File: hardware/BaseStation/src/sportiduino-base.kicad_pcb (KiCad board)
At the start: 2 copper layers, 76.8 x 44.7 mm, 38 parts, among them SW1 SW_Reed, X1 Battery, X2 Prog, X3 RC522

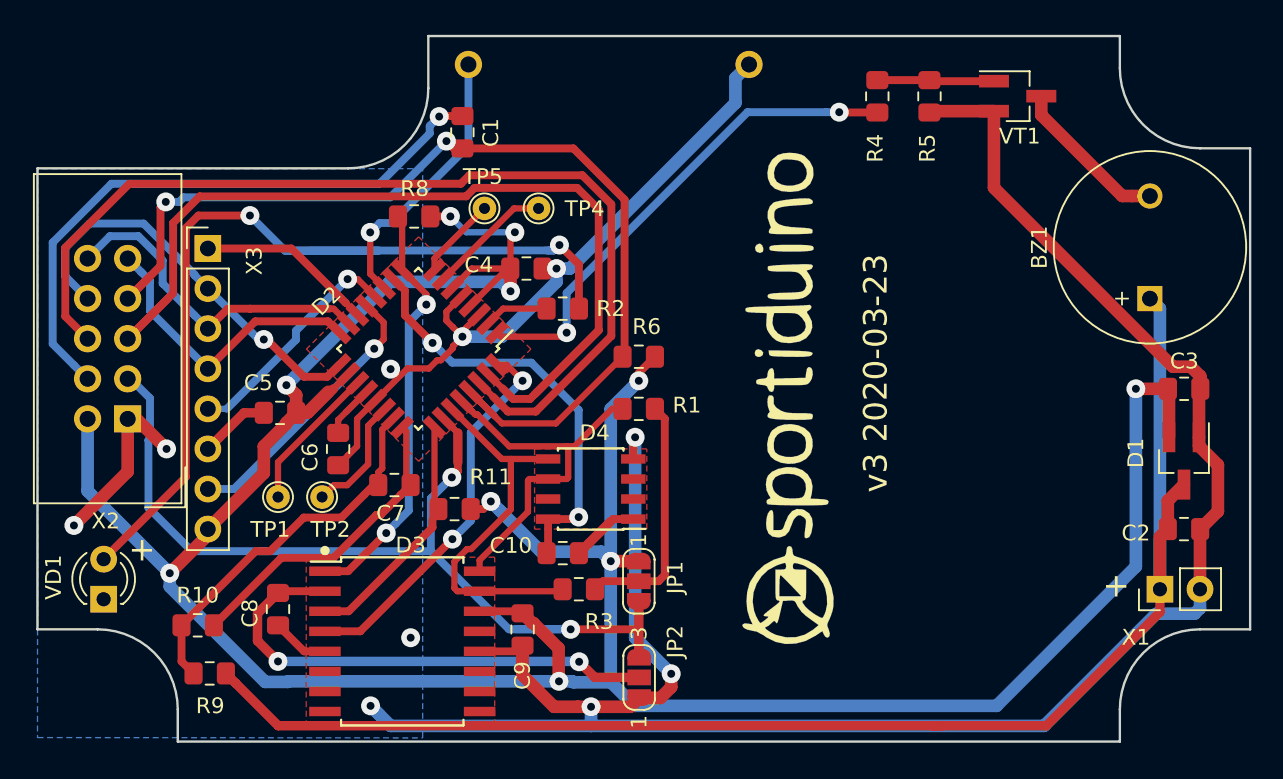
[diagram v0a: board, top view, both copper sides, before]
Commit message: New BS PCB v3 (2021-01-01)
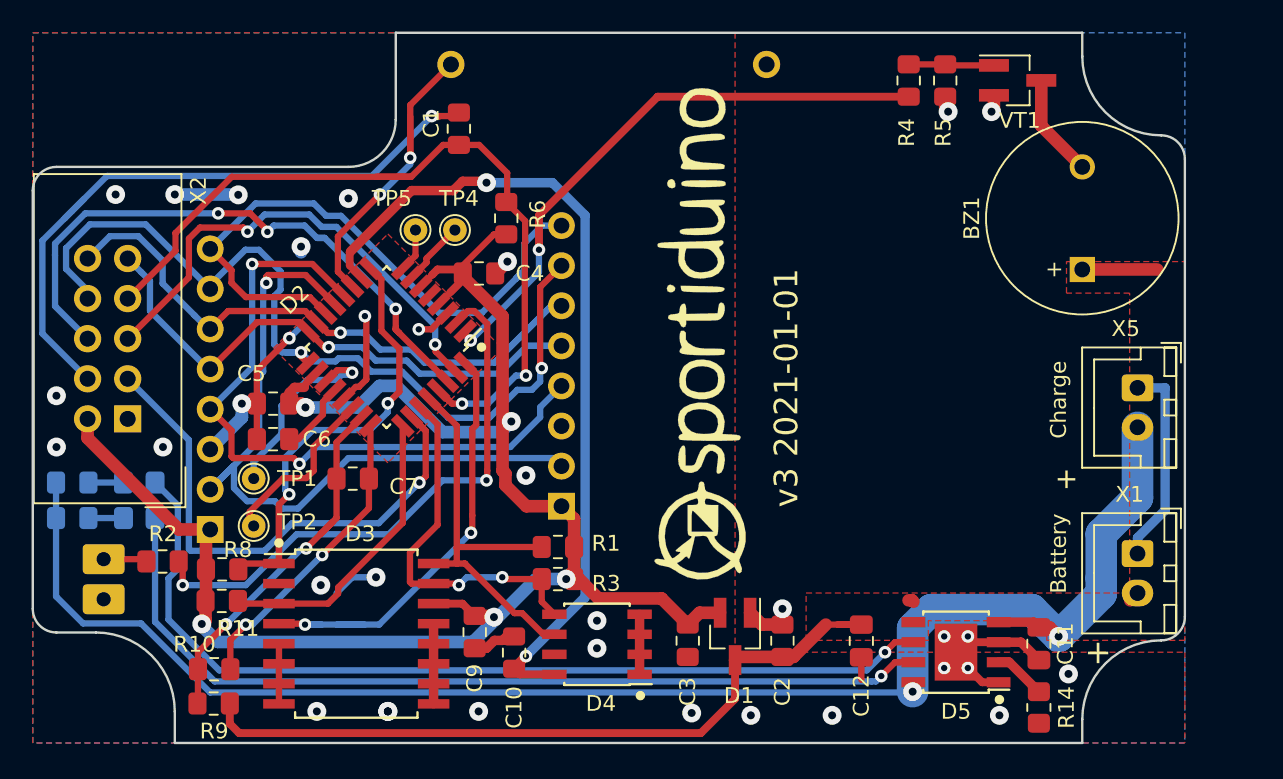
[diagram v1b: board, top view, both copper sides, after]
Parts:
- removed C8: 100 nF, Capacitor_SMD:C_0805_2012Metric_Pad1.15x1.40mm_HandSolder
- removed JP1, JP2: SolderJumper_3_Bridged12, Jumper:SolderJumper-3_P1.3mm_Open_RoundedPad1.0x1.5mm_NumberLabels
- added C11: 10 uF, Capacitor_SMD:C_0805_2012Metric_Pad1.18x1.45mm_HandSolder, F.Cu at (197.3, 97.2)
- added C12: 10 uF, Capacitor_SMD:C_0805_2012Metric_Pad1.18x1.45mm_HandSolder, F.Cu at (186.0, 97.0)
- added D5: TP4056, Sportiduino:TP4056_SOP-8-PP, F.Cu at (192.0, 97.7)
- added G***: LOGO, Sportiduino:logo, B.Cu at (165.5, 97.7)
- added R12: 1K, Resistor_SMD:R_0805_2012Metric_Pad1.20x1.40mm_HandSolder, B.Cu at (140.3, 86.9)
- added R13: 1K, Resistor_SMD:R_0805_2012Metric_Pad1.20x1.40mm_HandSolder, B.Cu at (140.3, 89.2)
- added R14: 3K3, Resistor_SMD:R_0805_2012Metric_Pad1.20x1.40mm_HandSolder, F.Cu at (197.3, 101.2)
- added VD2: 0805, LED_SMD:LED_0805_2012Metric_Pad1.15x1.40mm_HandSolder, B.Cu at (136.0, 86.9)
- added VD3: 0805, LED_SMD:LED_0805_2012Metric_Pad1.15x1.40mm_HandSolder, B.Cu at (136.0, 89.2)
- added X4: MINI RC522, Connector_PinHeader_2.54mm:PinHeader_1x08_P2.54mm_Vertical, B.Cu at (167.0, 88.4)
- added X5: Charge, Connector_JST:JST_XH_B2B-XH-A_1x02_P2.50mm_Vertical, F.Cu at (203.5, 80.9)
- VD1, X3: moved to B.Cu
- X1: footprint Connector_PinHeader_2.54mm:PinHeader_1x02_P2.54mm_Vertical -> Connector_JST:JST_XH_B2B-XH-A_1x02_P2.50mm_Vertical
- moved C3 35.3 mm to (175.0, 97.0), turned to 270 degrees
- moved D1 30.5 mm to (178.0, 96.7)
- moved R2 30.0 mm to (141.8, 91.9), turned to 0 degrees
- moved C2 26.4 mm to (181.0, 97.0), turned to 90 degrees
- moved R8 25.5 mm to (145.5, 92.4), turned to 0 degrees
- moved X3 17.8 mm to (144.8, 89.9)
- moved R11 15.9 mm to (145.5, 94.4), turned to 0 degrees
- moved R6 12.1 mm to (163.5, 70.2), turned to 90 degrees
- moved R1 10.1 mm to (166.8, 91.0)
- moved D4 9.85 mm to (169.3, 97.2)
- moved C10 7.01 mm to (164.0, 97.7), turned to 90 degrees
- moved G*** 6.91 mm to (175.8, 77.4)
- moved TP4 5.47 mm to (160.3, 70.9)
- moved TP2 4.71 mm to (147.5, 89.7)
- moved BZ1 4.67 mm to (200.0, 73.4)
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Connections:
- D3 pad 2: Net-(C8-Pad1) -> GNDD
- R1 pad 1: Net-(JP1-Pad2) -> +3V3
- R3 pad 1: Net-(JP1-Pad2) -> +3V3
- X1 pad 1: +BATT -> GNDD
- X1 pad 2: GNDD -> +BATT
- X3 pad 1: /PB2 -> +3V3
- X3 pad 2: PB5 -> /PB1
- X3 pad 3: PB3 -> GNDD
- X3 pad 4: PB4 -> /PB0
- X3 pad 5: /PB0 -> PB4
- X3 pad 6: GNDD -> PB3
- X3 pad 7: /PB1 -> PB5
- X3 pad 8: +3V3 -> /PB2
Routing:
- net GNDD: track 205.1 -> 72.1 mm, vias 10 -> 34
- net Net-(C11-Pad1): track 0.00 -> 98.0 mm, vias 0 -> 2
- net +3V3: track 202.4 -> 114.9 mm, vias 10 -> 5
- net Net-(D5-Pad6): track 0.00 -> 58.8 mm, vias 0 -> 1
- net Net-(R2-Pad1): track 59.5 -> 2.77 mm, vias 2 -> 0
- net Net-(D5-Pad7): track 0.00 -> 56.7 mm, vias 0 -> 1
- net TX: track 69.9 -> 31.0 mm, vias 0 -> 2
- net +BATT: track 91.7 -> 54.0 mm
- net /LED: track 4.10 -> 36.2 mm, vias 0 -> 2
- net Net-(C8-Pad1): track 31.7 -> 0.00 mm, vias 2 -> 0
- net /PB1: track 17.7 -> 49.1 mm
- net /PB2: track 11.2 -> 42.2 mm
- net /PB0: track 14.8 -> 45.3 mm, vias 1 -> 2
- net PB5: track 27.1 -> 56.4 mm, vias 1 -> 2
- net PC3: track 60.6 -> 34.6 mm, vias 2 -> 1
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- added copper zone on F.Cu, net +BATT
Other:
- board size 76.8 x 44.7 mm -> 73 x 45 mm
- net class Default: trace_width 0.5 -> 0.4; via_dia 1.2 -> 0.8; via_drill 0.5 -> 0.4
- rule via_min_size: 1.2 -> 0.8
- board text added: "Ali 83x58mm"
- board text added: "v3 2021-01-01"
- board text removed: "v3 2020-03-23"
